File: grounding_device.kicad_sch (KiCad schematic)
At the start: 161 parts, among them IC1 NE555P, IC2 NE555P, IC3 NE555P, IC4 NE555P, Q1 2N2222, Q10 2N2222, Q11 2N2222, Q12 2N2222, Q2 2N2222, Q3 2N2222, Q4 2N2222, Q5 2N2222, Q6 2N2222, Q7 2N2222, Q8 2N2222, Q9 2N2222

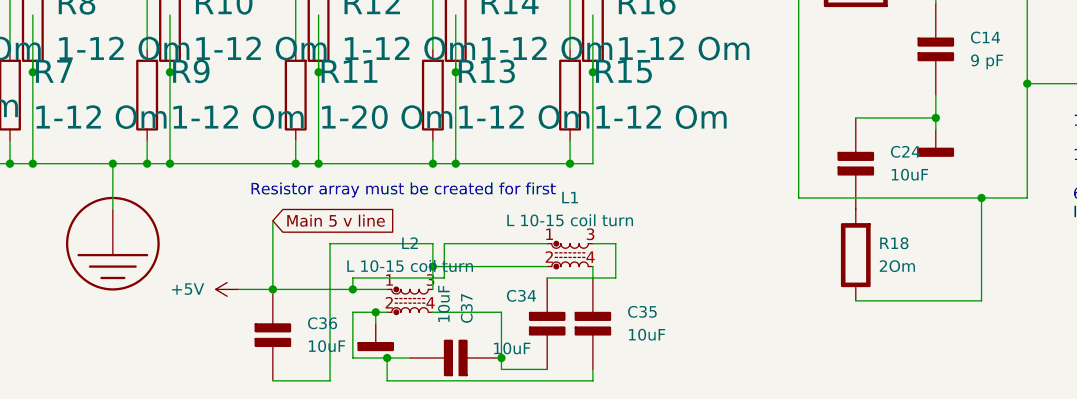
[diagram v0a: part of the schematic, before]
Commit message: Upgrade
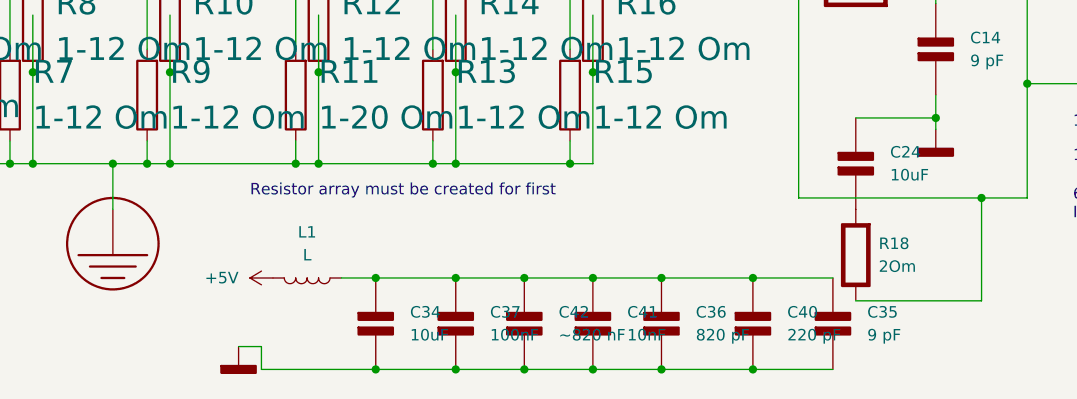
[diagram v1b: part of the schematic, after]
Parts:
- removed L1, L2: L 10-15 coil turn, symbol Device:L_Ferrite_Coupled_Small_1324
- added C40: 220 pF, symbol PCM_Elektuur:C
- added C41: 10nF, symbol PCM_Elektuur:C
- added C42: ~820 nF, symbol PCM_Elektuur:C
- added L1: L, symbol Device:L
- C35: value 10uF -> 9 pF
- C36: value 10uF -> 820 pF
- C37: value 10uF -> 100nF
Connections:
- net +5V: now also L1.2; no longer C36.1 (+)
- net 0: now also C34.2 (-), C36.2 (-), C40.2 (-), C41.2 (-), C42.2 (-)
- net at C35.1 (+): now also C34.1 (+), C36.1 (+), C37.1 (+), C40.1 (+), C41.1 (+), C42.1 (+), L1.1
